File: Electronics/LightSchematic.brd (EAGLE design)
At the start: 68.6 x 35.2 mm, 7 parts, among them IC1 7805T, IC2 ATMEGA328-20P

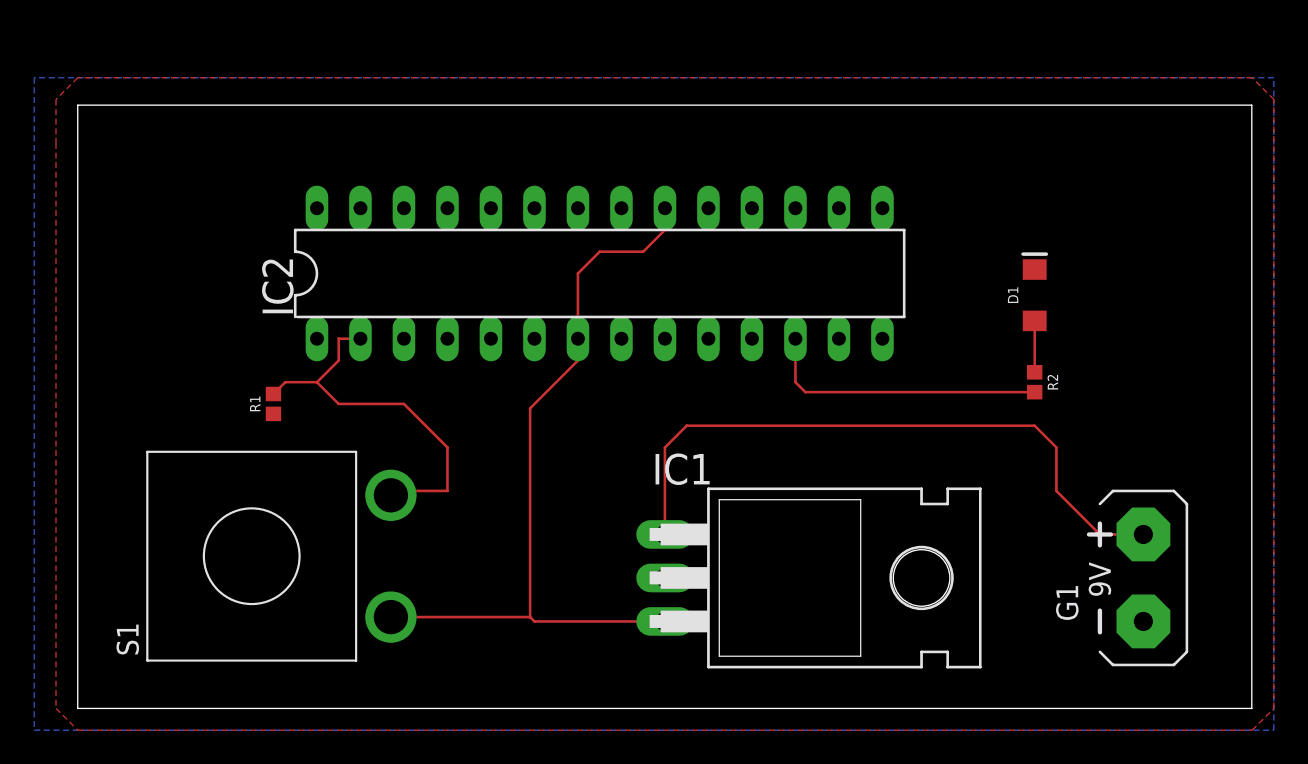
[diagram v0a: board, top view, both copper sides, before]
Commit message: Add v0.2.1 for milestone 4 review
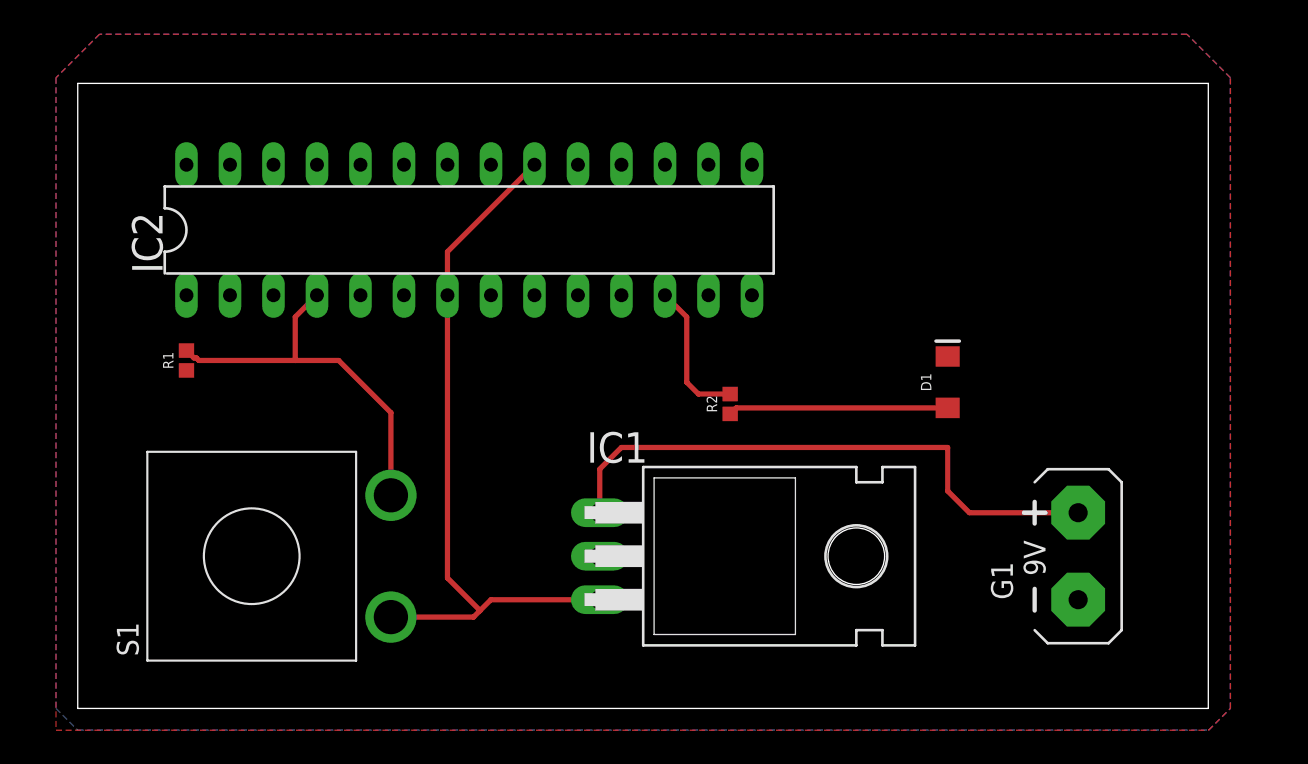
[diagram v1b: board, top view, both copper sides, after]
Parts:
- moved R2 17.8 mm to (38.1, 17.8), turned to 90 degrees
- moved IC2 8.03 mm to (22.9, 27.9)
- moved D1 7.18 mm to (50.8, 19.1)
- moved R1 5.68 mm to (6.35, 20.3)
- moved IC1 4.02 mm to (40.6, 8.89)
- moved G1 4.02 mm to (58.4, 8.89)
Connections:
- net DIN: now also IC2.4; no longer IC2.2
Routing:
- net N$3: track 3.00 -> 12.8 mm
- net PWM: track 16.8 -> 8.43 mm
- net 9V: track 37.7 -> 34.1 mm
- net 5V: track 44.7 -> 41.5 mm
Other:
- board size 68.6 x 35.2 mm -> 66 x 36.5 mm
